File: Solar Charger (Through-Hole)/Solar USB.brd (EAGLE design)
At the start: 74.6 x 24.1 mm, 22 parts, among them U1 MCP73871-2CCI/ML

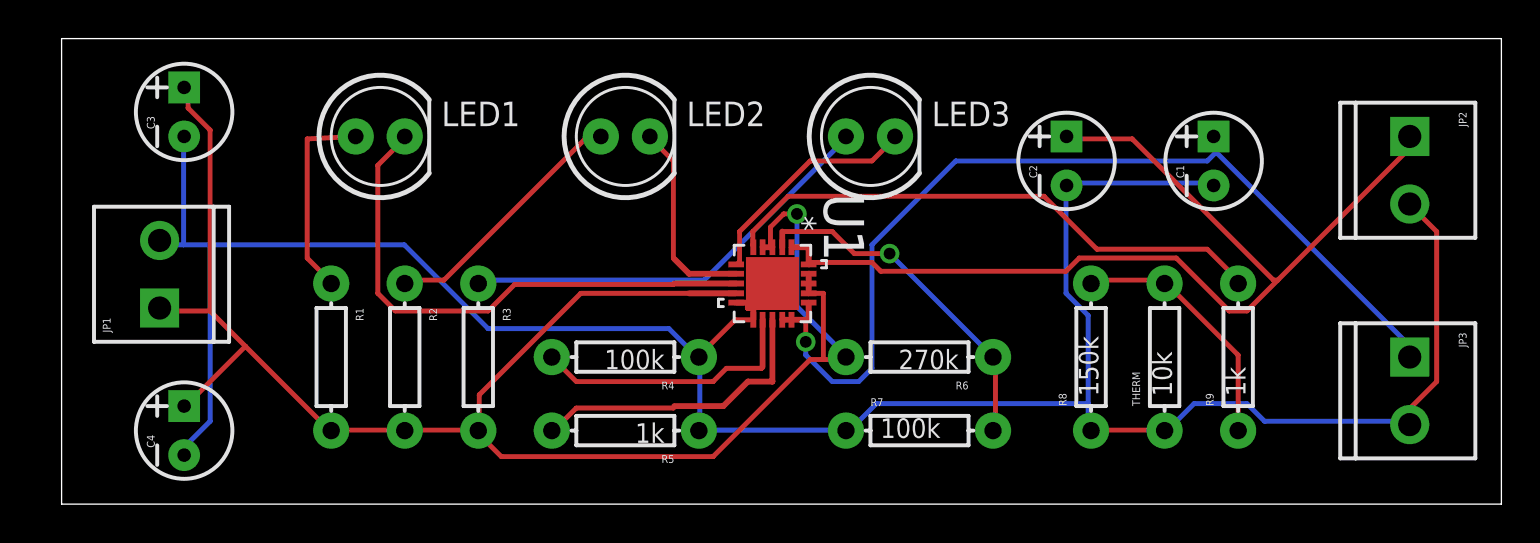
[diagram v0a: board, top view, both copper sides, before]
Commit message: boost
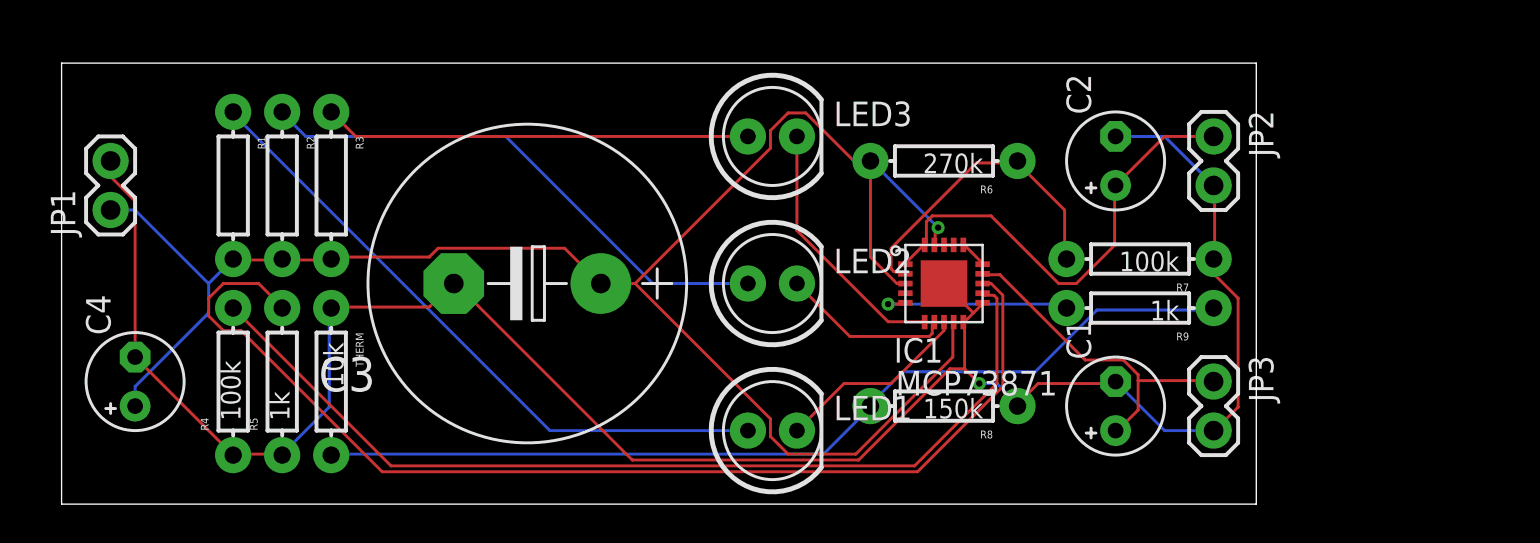
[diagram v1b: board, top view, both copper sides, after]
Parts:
- removed U1: MCP73871-2CCI/ML, Microchip_By_element14_Batch_1:QFN50P400X400X100-21N
- added IC1: MCP73871, adafruit:QFN20
- C1, C2, C4: device SparkFun-Capacitors:CPOL-RADIAL-10UF-25V-KIT -> adafruit:E2,5-5
- C3: device SparkFun-Capacitors:CPOL-RADIAL-10UF-25V-KIT -> adafruit:E7,5-16
- JP1, JP2, JP3: value M023.5MM -> M02PTH; device SparkFun-Connectors:SCREWTERMINAL-3.5MM-2 -> SparkFun-Connectors:1X02
- moved THERM 43.2 mm to (14.0, 6.35), turned to 270 degrees
- moved LED1 25.4 mm to (36.8, 3.81)
- moved R4 20.4 mm to (8.89, 6.35), turned to 90 degrees
- moved C3 19.9 mm to (24.1, 11.4), turned to 180 degrees
- moved R5 18.0 mm to (11.4, 6.35), turned to 90 degrees
- moved R7 14.5 mm to (55.9, 12.7), turned to 180 degrees
- moved C1 13.7 mm to (54.6, 5.08)
- moved R3 11.7 mm to (14.0, 16.5)
- moved R2 10.9 mm to (11.4, 16.5)
- moved LED2 10.8 mm to (36.8, 11.4)
- moved R1 10.2 mm to (8.89, 16.5)
- moved R6 10.2 mm to (45.7, 17.8)
- moved JP3 10.2 mm to (59.7, 6.35)
- moved JP2 10.2 mm to (59.7, 19.1)
- moved R8 8.03 mm to (45.7, 5.08), turned to 180 degrees
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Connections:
- removed net N$6: C1.1, JP3.1, U1.14, U1.15, U1.16
- removed net N$7: C2.1, JP2.1, U1.1, U1.20
- new net N$15: C2.+, IC1.1, IC1.20, JP2.1
- new net N$17: C1.+, IC1.14, IC1.15, IC1.16, JP3.1
- net N$1: now also IC1.6, LED3.K; no longer R9.P$2, U1.5
- net N$10: now also C3.+, C4.+, IC1.17, IC1.18, IC1.19, IC1.3, IC1.4, IC1.9; no longer C3.1, C4.1, U1.17, U1.18, U1.19, U1.3, U1.4, U1.9
- net N$11: now also IC1.5, R9.P$2; no longer LED1.K, U1.8
- net N$16: now also IC1.2; no longer U1.2
- net N$2: now also C1.-, C2.-, C3.-, C4.-, IC1.10, IC1.11, IC1.21; no longer C1.2, C2.2, C3.2, C4.2, U1.10, U1.11, U1.21
- net N$3: now also IC1.12; no longer U1.12
- net N$4: now also IC1.13; no longer U1.13
- net N$8: now also IC1.7, LED2.K; no longer LED3.K, U1.6
- net N$9: now also IC1.8, LED1.K; no longer LED2.K, U1.7
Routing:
- net N$7: track 52.7 -> 0.00 mm
- net N$6: track 51.1 -> 0.00 mm, vias 1 -> 0
- net N$4: track 15.7 -> 57.9 mm
- net N$3: track 14.2 -> 50.0 mm
- net N$5: track 13.3 -> 49.0 mm
- net N$15: track 0.00 -> 24.1 mm
- net N$12: track 10.5 -> 33.6 mm
- net N$2: track 130.9 -> 109.6 mm, vias 0 -> 1
- net N$17: track 0.00 -> 19.5 mm
- net N$11: track 28.2 -> 10.2 mm, vias 0 -> 1
- net N$1: track 28.7 -> 13.5 mm
- net N$13: track 13.3 -> 27.8 mm
- net N$10: track 91.9 -> 95.2 mm
- net N$8: track 11.9 -> 8.84 mm
- net N$16: track 18.4 -> 16.4 mm, vias 1 -> 0
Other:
- board size 74.6 x 24.1 mm -> 61.9 x 22.9 mm
